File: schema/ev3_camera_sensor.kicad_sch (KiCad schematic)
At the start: 13 parts, among them J1 OV7675 B0070, J2 WS2812B, J3 dry_cell_x2, J5 EV3_PORT_1, Q1 PMOS

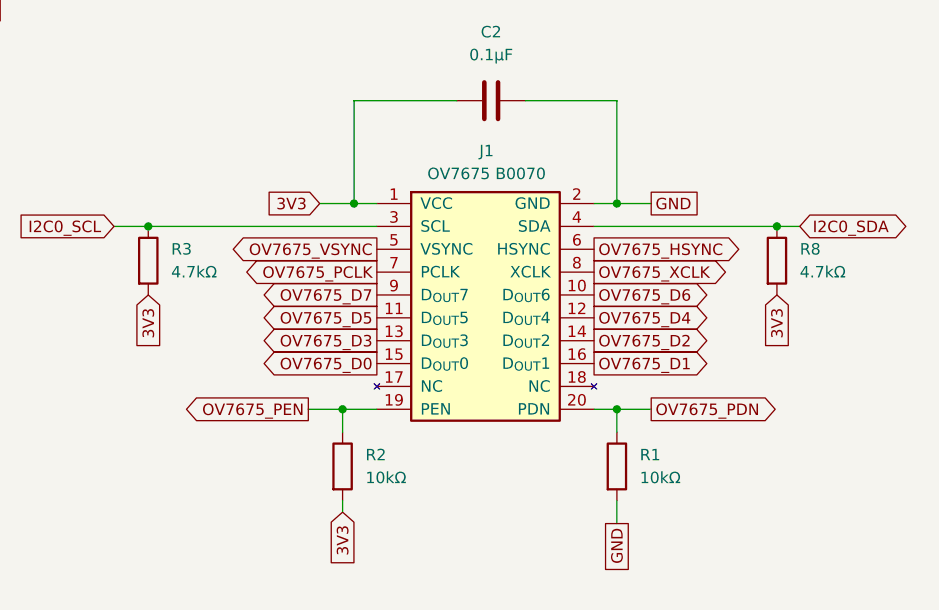
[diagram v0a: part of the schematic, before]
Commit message: Update Schema
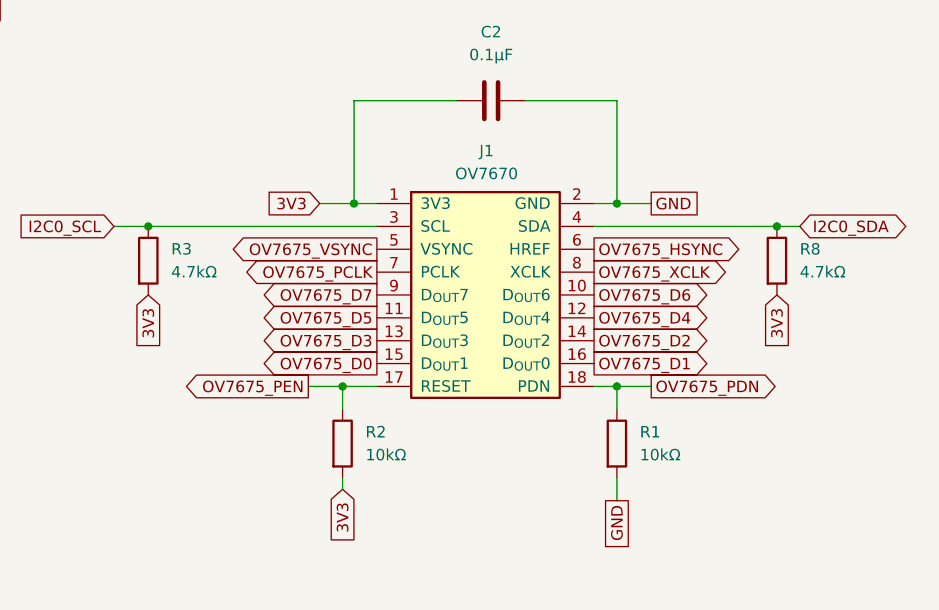
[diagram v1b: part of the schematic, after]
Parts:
- J1: value OV7675 B0070 -> OV7670
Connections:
- net OV7675_PDN: now also J1.18 (PDN); no longer J1.20 (PDN)
- net OV7675_PEN: now also J1.17 (RESET); no longer J1.19 (PEN)
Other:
- moved on the sheet: R1, R2
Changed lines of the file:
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@@
 	)
 	(junction
-		(at 236.22 137.16)
+		(at 236.22 134.62)
 		(diameter 0)
 		(color 0 0 0 0)
@@
 	)
 	(junction
-		(at 205.74 137.16)
+		(at 205.74 134.62)
 		(diameter 0)
 		(color 0 0 0 0)
@@
 	(wire
 		(pts
-			(xy 209.55 137.16) (xy 205.74 137.16)
-		)
-		(stroke
-			(width 0)
-			(type default)
-		)
-	)
-	(wire
-		(pts
-			(xy 236.22 149.86) (xy 236.22 147.32)
+			(xy 209.55 134.62) (xy 205.74 134.62)
+		)
+		(stroke
+			(width 0)
+			(type default)
+		)
+	)
+	(wire
+		(pts
+			(xy 236.22 147.32) (xy 236.22 144.78)
 		)
 		(stroke
@@
 	(wire
 		(pts
-			(xy 236.22 137.16) (xy 236.22 139.7)
+			(xy 236.22 134.62) (xy 236.22 137.16)
 		)
 		(stroke
@@
 	(wire
 		(pts
-			(xy 236.22 137.16) (xy 240.03 137.16)
-		)
-		(stroke
-			(width 0)
-			(type default)
-		)
-	)
-	(wire
-		(pts
-			(xy 233.68 137.16) (xy 236.22 137.16)
+			(xy 236.22 134.62) (xy 240.03 134.62)
+		)
+		(stroke
+			(width 0)
+			(type default)
+		)
+	)
+	(wire
+		(pts
+			(xy 233.68 134.62) (xy 236.22 134.62)
 		)
 		(stroke
@@
 	(wire
 		(pts
-			(xy 205.74 137.16) (xy 205.74 139.7)
+			(xy 205.74 134.62) (xy 205.74 137.16)
 		)
 		(stroke
@@
 	(wire
 		(pts
-			(xy 205.74 148.59) (xy 205.74 147.32)
+			(xy 205.74 146.05) (xy 205.74 144.78)
 		)
 		(stroke
@@
 	(wire
 		(pts
-			(xy 201.93 137.16) (xy 205.74 137.16)
+			(xy 201.93 134.62) (xy 205.74 134.62)
 		)
 		(stroke
@@
 	(global_label "3V3"
 		(shape input)
-		(at 205.74 148.59 270)
-		(fields_autoplaced yes)
-		(effects
-			(font
-				(size 1.27 1.27)
-			)
-			(justify right)
-		)
-		(property "Intersheetrefs" "${INTERSHEET_REFS}"
-			(at 205.74 155.0828 90)
+		(at 205.74 146.05 270)
+		(fields_autoplaced yes)
+		(effects
+			(font
+				(size 1.27 1.27)
+			)
+			(justify right)
+		)
+		(property "Intersheetrefs" "${INTERSHEET_REFS}"
+			(at 205.74 152.5428 90)
 			(hide yes)
 			(show_name no)
@@
 	(global_label "OV7675_PDN"
 		(shape output)
-		(at 240.03 137.16 0)
+		(at 240.03 134.62 0)
 		(fields_autoplaced yes)
 		(effects
@@
 		)
 		(property "Intersheetrefs" "${INTERSHEET_REFS}"
-			(at 255.1104 137.16 0)
+			(at 255.1104 134.62 0)
 			(hide yes)
 			(show_name no)
@@
 	(global_label "GND"
 		(shape passive)
-		(at 236.22 149.86 270)
-		(fields_autoplaced yes)
-		(effects
-			(font
-				(size 1.27 1.27)
-			)
-			(justify right)
-		)
-		(property "Intersheetrefs" "${INTERSHEET_REFS}"
-			(at 236.22 155.6044 90)
+		(at 236.22 147.32 270)
+		(fields_autoplaced yes)
+		(effects
+			(font
+				(size 1.27 1.27)
+			)
+			(justify right)
+		)
+		(property "Intersheetrefs" "${INTERSHEET_REFS}"
+			(at 236.22 153.0644 90)
 			(hide yes)
 			(show_name no)
@@
 	(global_label "OV7675_PEN"
 		(shape output)
-		(at 201.93 137.16 180)
-		(fields_autoplaced yes)
-		(effects
-			(font
-				(size 1.27 1.27)
-			)
-			(justify right)
-		)
-		(property "Intersheetrefs" "${INTERSHEET_REFS}"
-			(at 186.9706 137.16 0)
+		(at 201.93 134.62 180)
+		(fields_autoplaced yes)
+		(effects
+			(font
+				(size 1.27 1.27)
+			)
+			(justify right)
+		)
+		(property "Intersheetrefs" "${INTERSHEET_REFS}"
+			(at 186.9706 134.62 0)
 			(hide yes)
 			(show_name no)
@@
 			)
 		)
-		(property "Value" "OV7675 B0070"
+		(property "Value" "OV7670"
 			(at 221.742 110.998 0)
 			(show_name no)
@@
 		)
 		(pin "17"
-		)
-		(pin "19"
-		)
-		(pin "20"
 		)
 		(pin "8"
@@
 	(symbol
 		(lib_id "Device:R")
-		(at 205.74 143.51 0)
+		(at 205.74 140.97 0)
 		(unit 1)
 		(body_style 1)
@@
 		(fields_autoplaced yes)
 		(property "Reference" "R2"
+			(at 208.28 139.6999 0)
+			(show_name no)
+			(do_not_autoplace no)
+			(effects
+				(font
+					(size 1.27 1.27)
+				)
+				(justify left)
+			)
+		)
+		(property "Value" "10kΩ"
 			(at 208.28 142.2399 0)
 			(show_name no)
@@
 			)
 		)
-		(property "Value" "10kΩ"
-			(at 208.28 144.7799 0)
-			(show_name no)
-			(do_not_autoplace no)
-			(effects
-				(font
-					(size 1.27 1.27)
-				)
-				(justify left)
-			)
-		)
 		(property "Footprint" ""
-			(at 203.962 143.51 90)
+			(at 203.962 140.97 90)
 			(hide yes)
 			(show_name no)
@@
 		)
 		(property "Datasheet" ""
-			(at 205.74 143.51 0)
+			(at 205.74 140.97 0)
 			(hide yes)
 			(show_name no)
@@
 		)
 		(property "Description" "Resistor"
-			(at 205.74 143.51 0)
+			(at 205.74 140.97 0)
 			(hide yes)
 			(show_name no)
@@
 	(symbol
 		(lib_id "Device:R")
-		(at 236.22 143.51 0)
+		(at 236.22 140.97 0)
 		(unit 1)
 		(body_style 1)
@@
 		(fields_autoplaced yes)
 		(property "Reference" "R1"
+			(at 238.76 139.6999 0)
+			(show_name no)
+			(do_not_autoplace no)
+			(effects
+				(font
+					(size 1.27 1.27)
+				)
+				(justify left)
+			)
+		)
+		(property "Value" "10kΩ"
 			(at 238.76 142.2399 0)
 			(show_name no)
@@
 			)
 		)
-		(property "Value" "10kΩ"
-			(at 238.76 144.7799 0)
-			(show_name no)
-			(do_not_autoplace no)
-			(effects
-				(font
-					(size 1.27 1.27)
-				)
-				(justify left)
-			)
-		)
 		(property "Footprint" ""
-			(at 234.442 143.51 90)
+			(at 234.442 140.97 90)
 			(hide yes)
 			(show_name no)
@@
 		)
 		(property "Datasheet" ""
-			(at 236.22 143.51 0)
+			(at 236.22 140.97 0)
 			(hide yes)
 			(show_name no)
@@
 		)
 		(property "Description" "Resistor"
-			(at 236.22 143.51 0)
-			(hide yes)
-			(show_name no)
+			(at 236.22 140.97 0)
+			(hide yes)
+			(show_name no)
